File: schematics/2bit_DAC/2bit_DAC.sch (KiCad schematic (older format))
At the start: 4 parts, among them U1 PORT

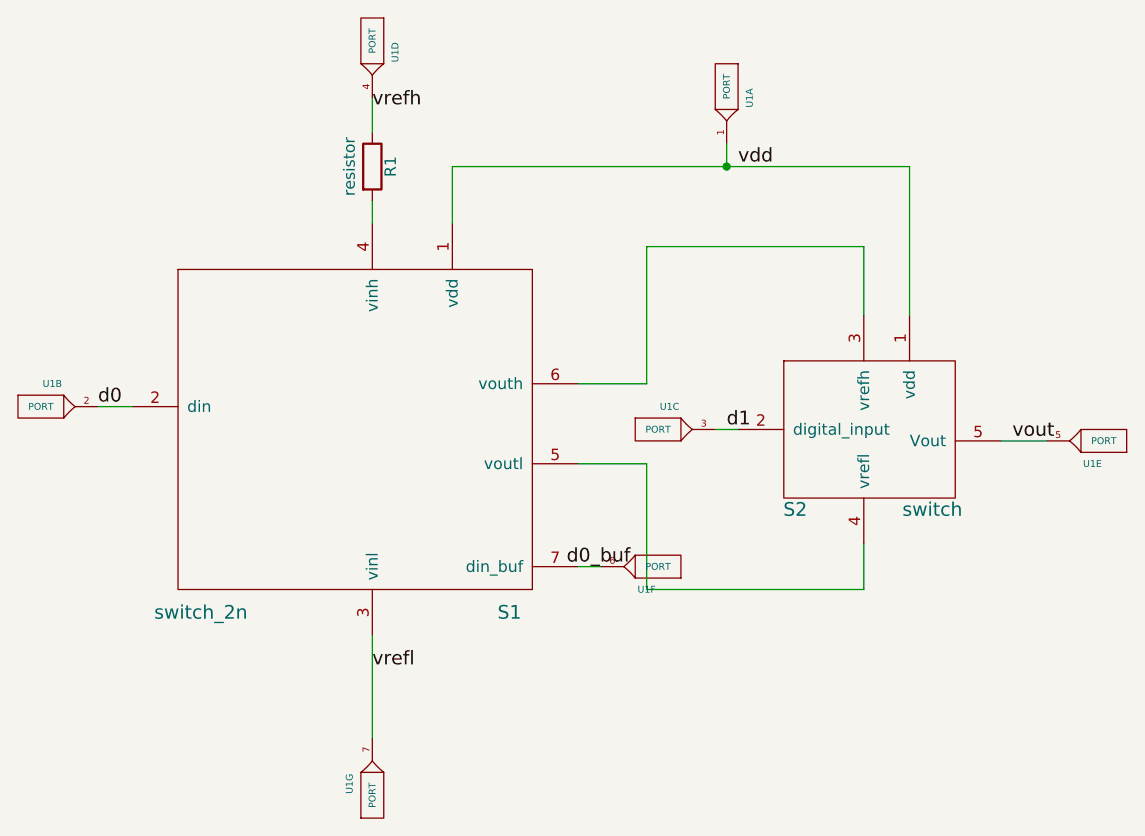
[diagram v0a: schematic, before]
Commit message: update
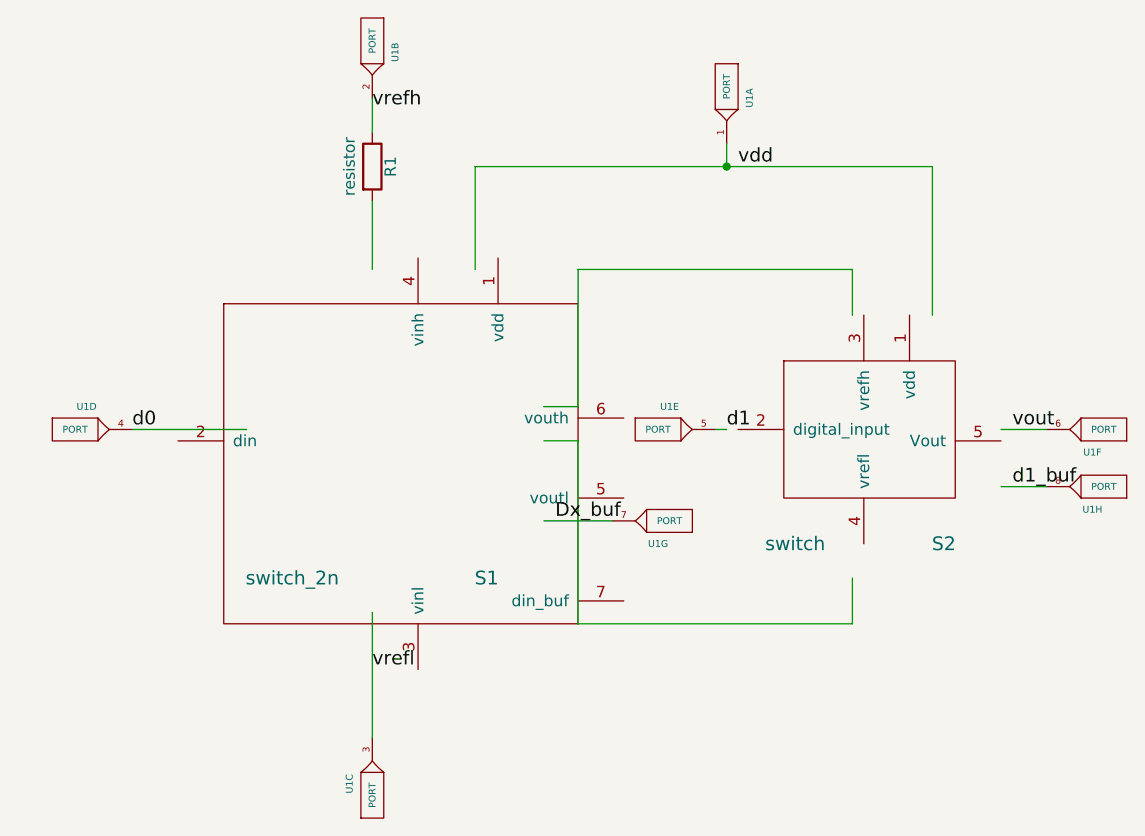
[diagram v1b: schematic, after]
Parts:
- added unit 8 of U1
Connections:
- net labels added: Dx_buf, d1_buf
- net labels removed: d0_buf
- wire segments 19 -> 20
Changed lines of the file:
@@
 EESchema Schematic File Version 2
+LIBS:eSim_Subckt
 LIBS:adc-dac
 LIBS:memory
@@
 LIBS:eSim_Power
 LIBS:eSim_Sources
-LIBS:eSim_Subckt
 LIBS:eSim_Nghdl
 LIBS:eSim_Ngveri
@@
 $Comp
 L PORT U1
-U 4 1 643E4B11
+U 2 1 643E4B11
 P 4750 2300
 F 0 "U1" H 4800 2400 30  0000 C CNN
@@
 F 2 "" H 4750 2300 60  0000 C CNN
 F 3 "" H 4750 2300 60  0000 C CNN
-	4    4750 2300
+	2    4750 2300
 	0    1    1    0
 $EndComp
@@
 $EndComp
 $Comp
-L switch_2n S1
-U 1 1 6443803F
-P 4650 3950
-F 0 "S1" H 5350 3100 60  0000 C CNN
-F 1 "switch_2n" H 4000 3100 60  0000 C CNN
-F 2 "" H 4750 4150 60  0001 C CNN
-F 3 "" H 4750 4150 60  0001 C CNN
-	1    4650 3950
-	1    0    0    -1
-$EndComp
-$Comp
-L PORT U1
-U 2 1 6443832D
-P 3300 3900
-F 0 "U1" H 3350 4000 30  0000 C CNN
-F 1 "PORT" H 3300 3900 30  0000 C CNN
-F 2 "" H 3300 3900 60  0000 C CNN
-F 3 "" H 3300 3900 60  0000 C CNN
-	2    3300 3900
-	1    0    0    -1
-$EndComp
-$Comp
-L switch S2
-U 1 1 6443C8B2
-P 6950 4050
-F 0 "S2" H 6600 3750 60  0000 C CNN
-F 1 "switch" H 7200 3750 60  0000 C CNN
-F 2 "" H 6950 4050 60  0001 C CNN
-F 3 "" H 6950 4050 60  0001 C CNN
-	1    6950 4050
-	1    0    0    -1
-$EndComp
-$Comp
-L PORT U1
-U 3 1 6443C967
+L PORT U1
+U 4 1 6443832D
+P 3450 4000
+F 0 "U1" H 3500 4100 30  0000 C CNN
+F 1 "PORT" H 3450 4000 30  0000 C CNN
+F 2 "" H 3450 4000 60  0000 C CNN
+F 3 "" H 3450 4000 60  0000 C CNN
+	4    3450 4000
+	1    0    0    -1
+$EndComp
+$Comp
+L PORT U1
+U 5 1 6443C967
 P 6000 4000
 F 0 "U1" H 6050 4100 30  0000 C CNN
@@
 F 2 "" H 6000 4000 60  0000 C CNN
 F 3 "" H 6000 4000 60  0000 C CNN
-	3    6000 4000
+	5    6000 4000
 	1    0    0    -1
 $EndComp
@@
 $Comp
 L PORT U1
-U 5 1 6443CA76
-P 7950 4050
-F 0 "U1" H 8000 4150 30  0000 C CNN
-F 1 "PORT" H 7950 4050 30  0000 C CNN
-F 2 "" H 7950 4050 60  0000 C CNN
-F 3 "" H 7950 4050 60  0000 C CNN
-	5    7950 4050
+U 6 1 6443CA76
+P 7950 4000
+F 0 "U1" H 8000 4100 30  0000 C CNN
+F 1 "PORT" H 7950 4000 30  0000 C CNN
+F 2 "" H 7950 4000 60  0000 C CNN
+F 3 "" H 7950 4000 60  0000 C CNN
+	6    7950 4000
 	-1   0    0    1
 $EndComp
-Text Label 3550 3900 0    60   ~ 0
+Text Label 3700 4000 0    60   ~ 0
 d0
 Text Label 6300 4000 0    60   ~ 0
 d1
-Text Label 7550 4050 0    60   ~ 0
+Text Label 7550 4000 0    60   ~ 0
 vout
 Text Label 6350 2850 0    60   ~ 0
@@
 $Comp
 L PORT U1
-U 6 1 6443CD41
-P 6000 4600
-F 0 "U1" H 6050 4700 30  0000 C CNN
-F 1 "PORT" H 6000 4600 30  0000 C CNN
-F 2 "" H 6000 4600 60  0000 C CNN
-F 3 "" H 6000 4600 60  0000 C CNN
-	6    6000 4600
+U 7 1 6443CD41
+P 6050 4400
+F 0 "U1" H 6100 4500 30  0000 C CNN
+F 1 "PORT" H 6050 4400 30  0000 C CNN
+F 2 "" H 6050 4400 60  0000 C CNN
+F 3 "" H 6050 4400 60  0000 C CNN
+	7    6050 4400
 	-1   0    0    1
 $EndComp
-Text Label 5600 4600 0    60   ~ 0
-d0_buf
 Wire Wire Line
 	4750 2550 4750 2700
 Wire Wire Line
-	4750 3000 4750 3100
-Wire Wire Line
-	3550 3900 3700 3900
-Wire Wire Line
-	5650 3800 5950 3800
-Wire Wire Line
-	5950 3800 5950 3200
-Wire Wire Line
-	5950 3200 6900 3200
-Wire Wire Line
-	6900 3200 6900 3500
-Wire Wire Line
-	5650 4150 5950 4150
-Wire Wire Line
-	5950 4150 5950 4700
-Wire Wire Line
-	5950 4700 6900 4700
-Wire Wire Line
-	6900 4700 6900 4500
-Wire Wire Line
-	5100 3100 5100 2850
-Wire Wire Line
-	5100 2850 7100 2850
-Wire Wire Line
-	7100 2850 7100 3500
+	4750 3000 4750 3300
+Wire Wire Line
+	3700 4000 4200 4000
 Wire Wire Line
 	6300 2750 6300 2850
 Connection ~ 6300 2850
 Wire Wire Line
-	6250 4000 6350 4000
-Wire Wire Line
-	7700 4050 7500 4050
-Wire Wire Line
-	5750 4600 5650 4600
-Wire Wire Line
-	4750 4900 4750 5350
+	4750 4800 4750 5350
 Text Label 4750 5050 0    60   ~ 0
 vrefl
 $Comp
 L PORT U1
-U 7 1 6443D6A0
+U 3 1 6443D6A0
 P 4750 5600
 F 0 "U1" H 4800 5700 30  0000 C CNN
@@
 F 2 "" H 4750 5600 60  0000 C CNN
 F 3 "" H 4750 5600 60  0000 C CNN
-	7    4750 5600
+	3    4750 5600
 	0    -1   -1   0
 $EndComp
+$Comp
+L PORT U1
+U 8 1 644BA624
+P 7950 4250
+F 0 "U1" H 8000 4350 30  0000 C CNN
+F 1 "PORT" H 7950 4250 30  0000 C CNN
+F 2 "" H 7950 4250 60  0000 C CNN
+F 3 "" H 7950 4250 60  0000 C CNN
+	8    7950 4250
+	-1   0    0    1
+$EndComp
+Text Label 7550 4250 0    60   ~ 0
+d1_buf
+$Comp
+L switch_2n S1
+U 1 1 644D50D8
+P 4850 4100
+F 0 "S1" H 5250 3550 60  0000 C CNN
+F 1 "switch_2n" H 4400 3550 60  0000 C CNN
+F 2 "" H 4850 4100 60  0001 C CNN
+F 3 "" H 4850 4100 60  0001 C CNN
+	1    4850 4100
+	1    0    0    -1
+$EndComp
+Wire Wire Line
+	5500 4050 5650 4050
+Wire Wire Line
+	5650 4050 5650 4850
+Wire Wire Line
+	5650 4850 6850 4850
+Wire Wire Line
+	6850 4850 6850 4650
+Wire Wire Line
+	5500 3900 5650 3900
+Wire Wire Line
+	5650 3900 5650 3300
+Wire Wire Line
+	5650 3300 6850 3300
+Wire Wire Line
+	6850 3300 6850 3500
+Wire Wire Line
+	5200 3300 5200 2850
+Wire Wire Line
+	5200 2850 7200 2850
+Wire Wire Line
+	7200 2850 7200 3500
+Wire Wire Line
+	6250 4000 6300 4000
+Wire Wire Line
+	7700 4000 7500 4000
+Wire Wire Line
+	7700 4250 7500 4250
+$Comp
+L switch S2
+U 1 1 644D5525
+P 6950 4050
+F 0 "S2" H 7250 3600 60  0000 C CNN
+F 1 "switch" H 6600 3600 60  0000 C CNN
+F 2 "" H 6850 4050 60  0001 C CNN
+F 3 "" H 6850 4050 60  0001 C CNN
+	1    6950 4050
+	1    0    0    -1
+$EndComp
+Wire Wire Line
+	5800 4400 5500 4400
+Text Label 5550 4400 0    60   ~ 0
+Dx_buf
 $EndSCHEMATC
